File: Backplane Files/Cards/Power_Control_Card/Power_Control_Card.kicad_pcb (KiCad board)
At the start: 2 copper layers, 100 x 62.5 mm, 17 parts, among them J1 Conn_01x02, Q1 FQPF27P06

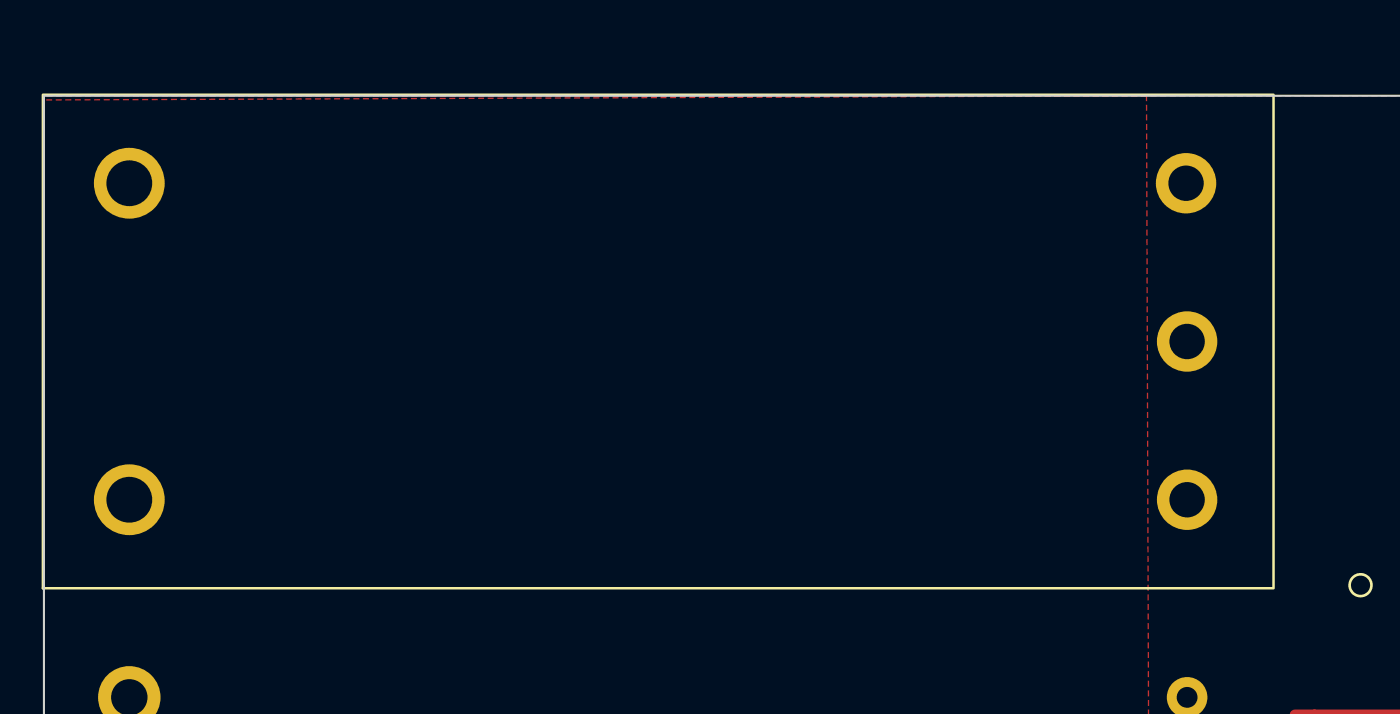
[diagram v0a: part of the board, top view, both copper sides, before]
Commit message: new power board
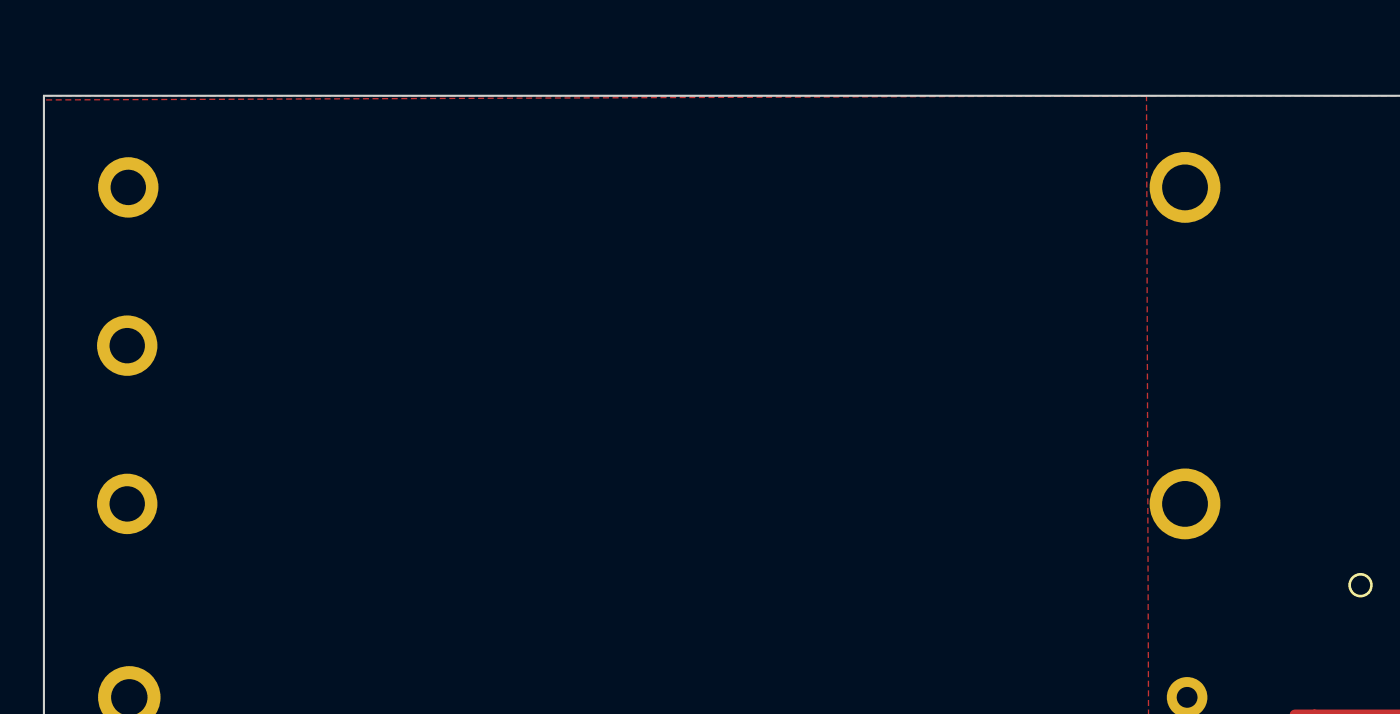
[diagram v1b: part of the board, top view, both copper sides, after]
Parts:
- U1: moved to B.Cu
- moved U1 50.9 mm to (154.1, 68.6)
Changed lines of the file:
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@@
 		)
 	)
-	(footprint "Custom:240W_CONV"
-		(layer "F.Cu")
-		(at 205 68.4 90)
-		(property "Reference" "U1"
-			(at 8.8392 -10.7188 90)
-			(unlocked yes)
-			(layer "F.SilkS")
-			(hide yes)
-			(effects
-				(font
-					(size 1 1)
-					(thickness 0.15)
-				)
-			)
-		)
-		(property "Value" "~"
-			(at 8.4328 -15.2908 90)
-			(unlocked yes)
-			(layer "F.Fab")
-			(hide yes)
-			(effects
-				(font
-					(size 1 1)
-					(thickness 0.15)
-				)
-			)
-		)
-		(property "Footprint" "Custom:240W_CONV"
-			(at 0 0 90)
-			(layer "F.Fab")
-			(hide yes)
-			(effects
-				(font
-					(size 1.27 1.27)
-					(thickness 0.15)
-				)
-			)
-		)
-		(property "Datasheet" ""
-			(at 0 0 90)
-			(layer "F.Fab")
-			(hide yes)
-			(effects
-				(font
-					(size 1.27 1.27)
-					(thickness 0.15)
-				)
-			)
-		)
-		(property "Description" ""
-			(at 0 0 90)
-			(layer "F.Fab")
-			(hide yes)
-			(effects
-				(font
-					(size 1.27 1.27)
-					(thickness 0.15)
-				)
-			)
-		)
-		(sheetname "Root")
-		(sheetfile "Power_Control_Card.kicad_sch")
-		(attr through_hole)
-		(fp_rect
-			(start -4.25 -54.95)
-			(end 19.45 4.15)
-			(stroke
-				(width 0.12)
-				(type default)
-			)
-			(fill none)
-			(layer "F.SilkS")
-		)
-		(pad "1" thru_hole circle
-			(at 0 0 90)
-			(size 2.9 2.9)
-			(drill 1.7)
-			(layers "*.Cu" "*.Mask")
-			(remove_unused_layers no)
-			(net 1 "/V_POWER")
-			(pinfunction "VIN")
-			(pintype "power_in")
-		)
-		(pad "2" thru_hole circle
-			(at 7.6 0 90)
-			(size 2.9 2.9)
-			(drill 1.7)
-			(layers "*.Cu" "*.Mask")
-			(remove_unused_layers no)
-			(net 33 "unconnected-(U1-RC-Pad2)")
-			(pinfunction "RC")
-			(pintype "input")
-		)
-		(pad "3" thru_hole circle
-			(at 15.2 -0.0508 90)
-			(size 2.9 2.9)
-			(drill 1.7)
-			(layers "*.Cu" "*.Mask")
-			(remove_unused_layers no)
-			(net 20 "SW1")
-			(pinfunction "IN-")
-			(pintype "power_in")
-		)
-		(pad "4" thru_hole circle
-			(at 15.2 -50.8 90)
-			(size 3.4 3.4)
-			(drill 2.2)
-			(layers "*.Cu" "*.Mask")
-			(remove_unused_layers no)
-			(net 20 "SW1")
-			(pinfunction "OUT-")
-			(pintype "power_out")
-		)
-		(pad "8" thru_hole circle
-			(at 0 -50.8 90)
-			(size 3.4 3.4)
-			(drill 2.2)
-			(layers "*.Cu" "*.Mask")
-			(remove_unused_layers no)
-			(net 5 "+12V")
-			(pinfunction "VOUT")
-			(pintype "power_out")
-		)
-	)
 	(footprint "Capacitor_SMD:C_0805_2012Metric_Pad1.18x1.45mm_HandSolder"
 		(layer "F.Cu")
@@
 		)
 	)
+	(footprint "Custom:240W_CONV"
+		(layer "B.Cu")
+		(at 154.1 68.6 90)
+		(property "Reference" "U1"
+			(at 8.8392 10.7188 -90)
+			(unlocked yes)
+			(layer "B.SilkS")
+			(hide yes)
+			(effects
+				(font
+					(size 1 1)
+					(thickness 0.15)
+				)
+				(justify mirror)
+			)
+		)
+		(property "Value" "~"
+			(at 8.4328 15.2908 -90)
+			(unlocked yes)
+			(layer "B.Fab")
+			(hide yes)
+			(effects
+				(font
+					(size 1 1)
+					(thickness 0.15)
+				)
+				(justify mirror)
+			)
+		)
+		(property "Footprint" "Custom:240W_CONV"
+			(at 0 0 90)
+			(layer "B.Fab")
+			(hide yes)
+			(effects
+				(font
+					(size 1.27 1.27)
+					(thickness 0.15)
+				)
+				(justify mirror)
+			)
+		)
+		(property "Datasheet" ""
+			(at 0 0 90)
+			(layer "B.Fab")
+			(hide yes)
+			(effects
+				(font
+					(size 1.27 1.27)
+					(thickness 0.15)
+				)
+				(justify mirror)
+			)
+		)
+		(property "Description" ""
+			(at 0 0 90)
+			(layer "B.Fab")
+			(hide yes)
+			(effects
+				(font
+					(size 1.27 1.27)
+					(thickness 0.15)
+				)
+				(justify mirror)
+			)
+		)
+		(sheetname "Root")
+		(sheetfile "Power_Control_Card.kicad_sch")
+		(attr through_hole)
+		(fp_rect
+			(start -4.25 54.95)
+			(end 19.45 -4.15)
+			(stroke
+				(width 0.12)
+				(type default)
+			)
+			(fill none)
+			(layer "B.SilkS")
+		)
+		(pad "1" thru_hole circle
+			(at 0 0 90)
+			(size 2.9 2.9)
+			(drill 1.7)
+			(layers "*.Cu" "*.Mask")
+			(remove_unused_layers no)
+			(net 1 "/V_POWER")
+			(pinfunction "VIN")
+			(pintype "power_in")
+		)
+		(pad "2" thru_hole circle
+			(at 7.6 0 90)
+			(size 2.9 2.9)
+			(drill 1.7)
+			(layers "*.Cu" "*.Mask")
+			(remove_unused_layers no)
+			(net 33 "unconnected-(U1-RC-Pad2)")
+			(pinfunction "RC")
+			(pintype "input")
+		)
+		(pad "3" thru_hole circle
+			(at 15.2 0.0508 90)
+			(size 2.9 2.9)
+			(drill 1.7)
+			(layers "*.Cu" "*.Mask")
+			(remove_unused_layers no)
+			(net 20 "SW1")
+			(pinfunction "IN-")
+			(pintype "power_in")
+		)
+		(pad "4" thru_hole circle
+			(at 15.2 50.8 90)
+			(size 3.4 3.4)
+			(drill 2.2)
+			(layers "*.Cu" "*.Mask")
+			(remove_unused_layers no)
+			(net 20 "SW1")
+			(pinfunction "OUT-")
+			(pintype "power_out")
+		)
+		(pad "8" thru_hole circle
+			(at 0 50.8 90)
+			(size 3.4 3.4)
+			(drill 2.2)
+			(layers "*.Cu" "*.Mask")
+			(remove_unused_layers no)
+			(net 5 "+12V")
+			(pinfunction "VOUT")
+			(pintype "power_out")
+		)
+	)
